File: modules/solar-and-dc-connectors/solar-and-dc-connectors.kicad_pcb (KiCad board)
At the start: 2 copper layers, 20 x 30.5 mm, 3 parts, among them J1 S2B-PH-K-SLFSN, J2 54-00127

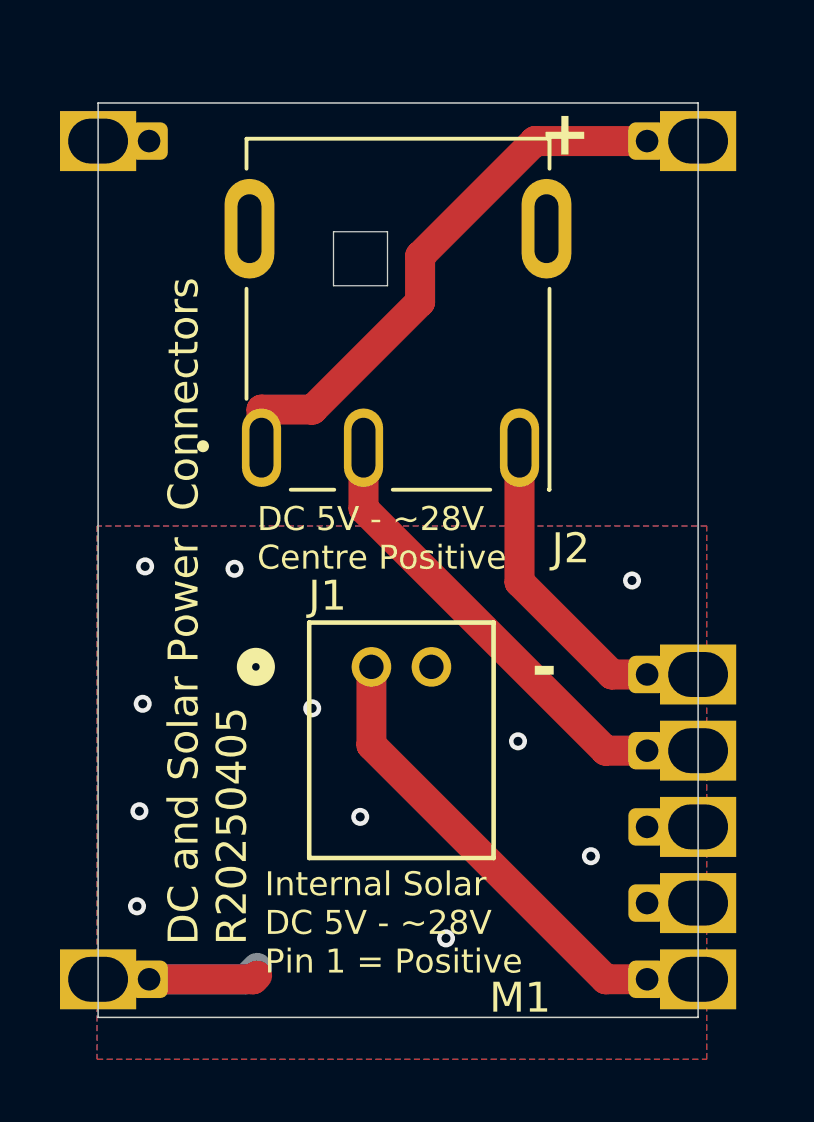
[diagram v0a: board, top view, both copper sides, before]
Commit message: Updating all modules
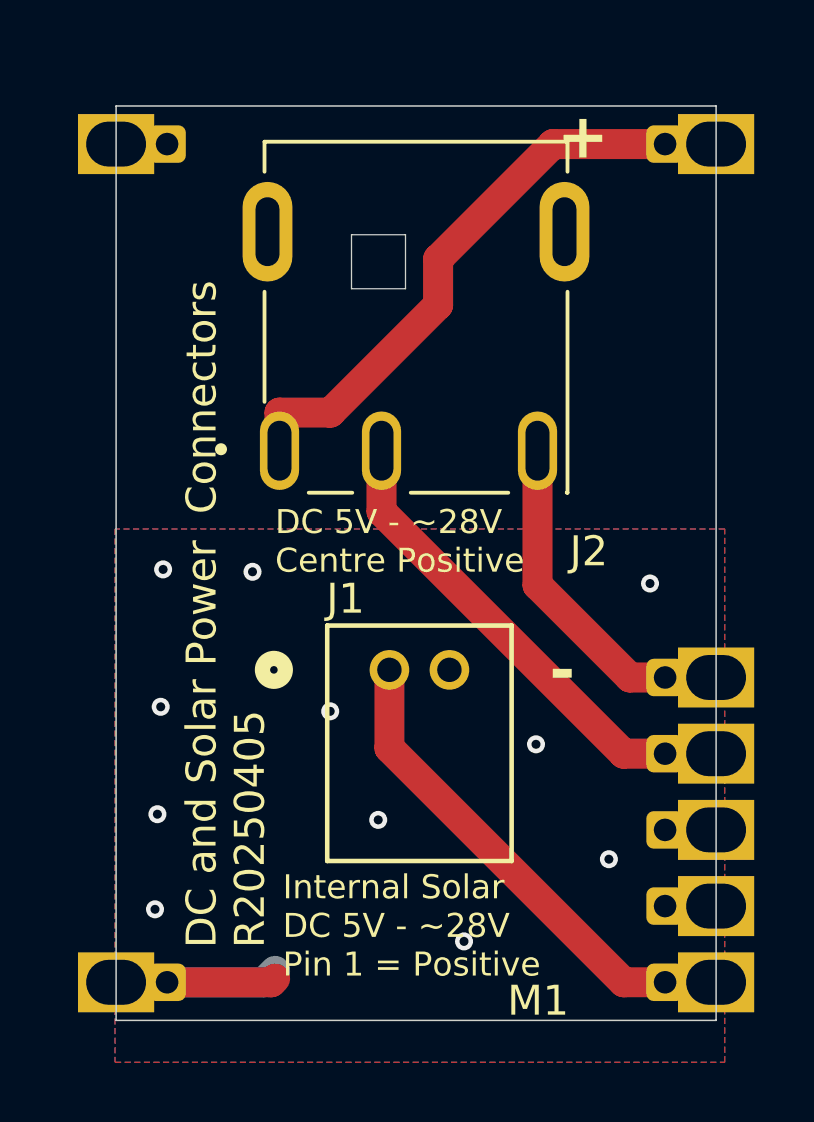
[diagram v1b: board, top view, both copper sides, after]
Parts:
- moved J1 0.61 mm to (63.1, 48.0)
- moved J2 0.61 mm to (64.0, 33.4)
- moved M1 0.61 mm to (64.0, 44.4)
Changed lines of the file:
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@@
 	(footprint "MegaCastle:CONN_S2B-PH-K-S_JST"
 		(layer "F.Cu")
-		(at 62.484 47.879)
+		(at 63.084 47.979)
 		(tags "S2B-PH-K-SLFSN ")
 		(property "Reference" "J1"
@@
 	(footprint "MegaCastle:MegaCastle2x12-Module-I20.0x25.7-M80181F-SPAREPAD"
 		(layer "F.Cu")
-		(at 63.373 44.323)
+		(at 63.973 44.423)
 		(property "Reference" "M1"
 			(at 4.067 14.587 0)
@@
 			(polygon
 				(pts
-					(xy 53.373 29.083) (xy 53.373 31.483) (xy 73.373 31.483) (xy 73.373 29.083)
+					(xy 53.973 29.183) (xy 53.973 31.583) (xy 73.973 31.583) (xy 73.973 29.183)
 				)
 			)
@@
 			(polygon
 				(pts
-					(xy 53.373 59.563) (xy 53.373 57.163) (xy 73.373 57.163) (xy 73.373 59.563)
+					(xy 53.973 59.663) (xy 53.973 57.263) (xy 73.973 57.263) (xy 73.973 59.663)
 				)
 			)
@@
 			(polygon
 				(pts
-					(xy 61.388759 30.631592) (xy 61.388759 29.163) (xy 65.392516 29.163) (xy 65.392516 30.631592)
+					(xy 61.988759 30.731592) (xy 61.988759 29.263) (xy 65.992516 29.263) (xy 65.992516 30.731592)
 				)
 			)
@@
 			(polygon
 				(pts
-					(xy 61.388759 58.014408) (xy 61.388759 59.483) (xy 65.392516 59.483) (xy 65.392516 58.014408)
+					(xy 61.988759 58.114408) (xy 61.988759 59.583) (xy 65.992516 59.583) (xy 65.992516 58.114408)
 				)
 			)
@@
 	(footprint "MegaCastle:TENSILITY_54-00127"
 		(layer "F.Cu")
-		(at 63.37 33.274 180)
+		(at 63.97 33.374 180)
 		(property "Reference" "J2"
 			(at -5.76 -10.656 180)
@@
 	)
 	(gr_text "-"
-		(at 67.818 48.768 0)
+		(at 68.418 48.868 0)
 		(layer "F.SilkS")
 		(effects
@@
 	)
 	(gr_text "DC and Solar Power  Connectors\nR20250405"
-		(at 58.42 57.15 90)
+		(at 59.02 57.25 90)
 		(layer "F.SilkS")
 		(effects
@@
 	)
 	(gr_text "+"
-		(at 68.072 30.988 0)
+		(at 68.672 31.088 0)
 		(layer "F.SilkS")
 		(effects
@@
 	)
 	(gr_text "DC 5V - ~28V\nCentre Positive"
-		(at 58.674 44.704 0)
+		(at 59.274 44.804 0)
 		(layer "F.SilkS")
 		(effects
@@
 	)
 	(gr_text "Internal Solar\nDC 5V - ~28V\nPin 1 = Positive\n"
-		(at 58.928 58.166 0)
+		(at 59.528 58.266 0)
 		(layer "F.SilkS")
 		(effects
@@
 	)
 	(gr_text "github.com/mega65/\n\nmegaphone-modular"
-		(at 65.024 57.15 -90)
+		(at 65.624 57.25 -90)
 		(layer "B.SilkS")
 		(effects
@@
 	)
 	(segment
-		(start 70.293 58.293)
-		(end 71.423 58.293)
+		(start 70.893 58.393)
+		(end 72.023 58.393)
 		(width 1)
 		(layer "F.Cu")
@@
 	)
 	(segment
-		(start 62.484 50.484)
-		(end 70.293 58.293)
+		(start 63.084 50.584)
+		(end 70.893 58.393)
 		(width 1)
 		(layer "F.Cu")
@@
 	)
 	(segment
-		(start 62.484 47.879)
-		(end 62.484 50.484)
+		(start 63.084 47.979)
+		(end 63.084 50.584)
 		(width 1)
 		(layer "F.Cu")
@@
 	)
 	(segment
-		(start 55.323 58.293)
-		(end 58.547 58.293)
-		(width 1)
-		(layer "F.Cu")
-		(net 5)
-	)
-	(segment
-		(start 58.547 58.293)
-		(end 58.674 58.166)
+		(start 55.923 58.393)
+		(end 59.147 58.393)
+		(width 1)
+		(layer "F.Cu")
+		(net 5)
+	)
+	(segment
+		(start 59.147 58.393)
+		(end 59.274 58.266)
 		(width 1)
 		(layer "F.Cu")
@@
 	)
 	(via
-		(at 64.97 56.93)
+		(at 65.57 57.03)
 		(size 0.6)
 		(drill 0.3)
@@
 	)
 	(via
-		(at 62.11 52.88)
+		(at 62.71 52.98)
 		(size 0.6)
 		(drill 0.3)
@@
 	)
 	(via
-		(at 69.8 54.19)
+		(at 70.4 54.29)
 		(size 0.6)
 		(drill 0.3)
@@
 	)
 	(via
-		(at 54.75 52.69)
+		(at 55.35 52.79)
 		(size 0.6)
 		(drill 0.3)
@@
 	)
 	(via
-		(at 54.94 44.53)
+		(at 55.54 44.63)
 		(size 0.6)
 		(drill 0.3)
@@
 	)
 	(via
-		(at 71.17 45)
+		(at 71.77 45.1)
 		(size 0.6)
 		(drill 0.3)
@@
 	)
 	(via
-		(at 57.92 44.61)
+		(at 58.52 44.71)
 		(size 0.6)
 		(drill 0.3)
@@
 	)
 	(via
-		(at 67.37 50.36)
+		(at 67.97 50.46)
 		(size 0.6)
 		(drill 0.3)
@@
 	)
 	(via
-		(at 54.86 49.11)
+		(at 55.46 49.21)
 		(size 0.6)
 		(drill 0.3)
@@
 	)
 	(via
-		(at 60.51 49.26)
+		(at 61.11 49.36)
 		(size 0.6)
 		(drill 0.3)
@@
 	)
 	(via
-		(at 54.67 55.86)
+		(at 55.27 55.96)
 		(size 0.6)
 		(drill 0.3)
@@
 	)
 	(segment
-		(start 55.323 58.293)
-		(end 58.293 58.293)
+		(start 55.923 58.393)
+		(end 58.893 58.393)
 		(width 1)
 		(layer "B.Cu")
@@
 	)
 	(segment
-		(start 58.293 58.293)
-		(end 58.674 57.912)
+		(start 58.893 58.393)
+		(end 59.274 58.012)
 		(width 1)
 		(layer "B.Cu")
@@
 	)
 	(segment
-		(start 64.107 35.715)
-		(end 64.107 34.183)
+		(start 64.707 35.815)
+		(end 64.707 34.283)
 		(width 1)
 		(layer "F.Cu")
@@
 	)
 	(segment
-		(start 64.107 34.183)
-		(end 67.937 30.353)
+		(start 64.707 34.283)
+		(end 68.537 30.453)
 		(width 1)
 		(layer "F.Cu")
@@
 	)
 	(segment
-		(start 60.518 39.304)
-		(end 64.107 35.715)
+		(start 61.118 39.404)
+		(end 64.707 35.815)
 		(width 1)
 		(layer "F.Cu")
@@
 	)
 	(segment
-		(start 58.82 39.304)
-		(end 60.518 39.304)
+		(start 59.42 39.404)
+		(end 61.118 39.404)
 		(width 1)
 		(layer "F.Cu")
@@
 	)
 	(segment
-		(start 67.937 30.353)
-		(end 71.423 30.353)
+		(start 68.537 30.453)
+		(end 72.023 30.453)
 		(width 1)
 		(layer "F.Cu")
@@
 	)
 	(segment
-		(start 58.82 40.574)
-		(end 58.82 39.304)
+		(start 59.42 40.674)
+		(end 59.42 39.404)
 		(width 1)
 		(layer "F.Cu")
@@
 	)
 	(segment
-		(start 70.503 48.133)
-		(end 71.423 48.133)
+		(start 71.103 48.233)
+		(end 72.023 48.233)
 		(width 1)
 		(layer "F.Cu")
@@
 	)
 	(segment
-		(start 67.42 40.574)
-		(end 67.42 45.05)
+		(start 68.02 40.674)
+		(end 68.02 45.15)
 		(width 1)
 		(layer "F.Cu")
@@
 	)
 	(segment
-		(start 67.42 45.05)
-		(end 70.503 48.133)
+		(start 68.02 45.15)
+		(end 71.103 48.233)
 		(width 1)
 		(layer "F.Cu")
@@
 	)
 	(segment
-		(start 70.293 50.673)
-		(end 71.423 50.673)
+		(start 70.893 50.773)
+		(end 72.023 50.773)
 		(width 1)
 		(layer "F.Cu")
@@
 	)
 	(segment
-		(start 62.22 40.574)
-		(end 62.22 42.6)
+		(start 62.82 40.674)
+		(end 62.82 42.7)
 		(width 1)
 		(layer "F.Cu")
@@
 	)
 	(segment
-		(start 62.22 42.6)
-		(end 70.293 50.673)
+		(start 62.82 42.7)
+		(end 70.893 50.773)
 		(width 1)
 		(layer "F.Cu")
@@
 		(polygon
 			(pts
-				(xy 53.34 43.18) (xy 53.34 60.96) (xy 73.66 60.96) (xy 73.66 43.18)
-			)
-		)
+				(xy 53.94 43.28) (xy 53.94 61.06) (xy 74.26 61.06) (xy 74.26 43.28)
+			)
+		)
